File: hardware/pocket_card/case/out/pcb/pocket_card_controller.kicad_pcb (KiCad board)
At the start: 2 copper layers, 80.5 x 37 mm, 19 parts, among them U1 SOIC-28W_7.5x17.9mm_P1.27mm

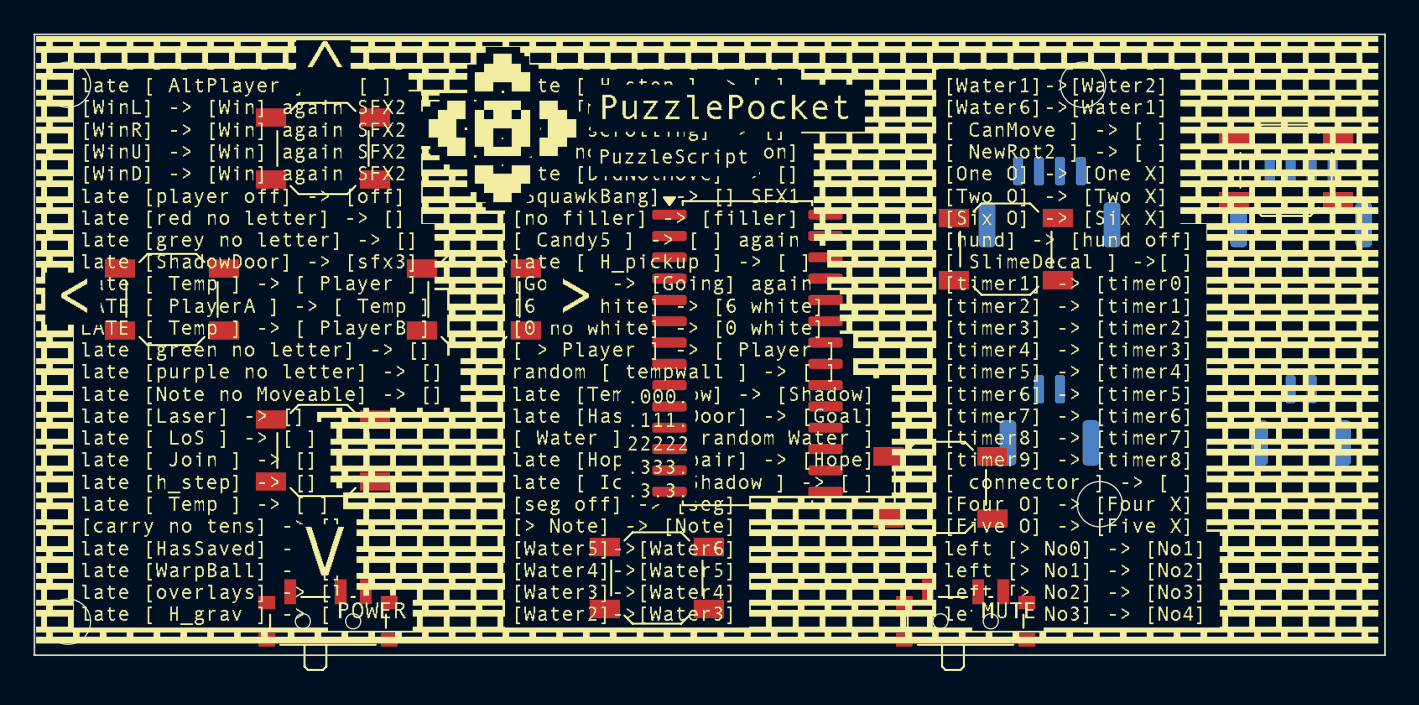
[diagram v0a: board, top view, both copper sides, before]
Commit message: regen pcb
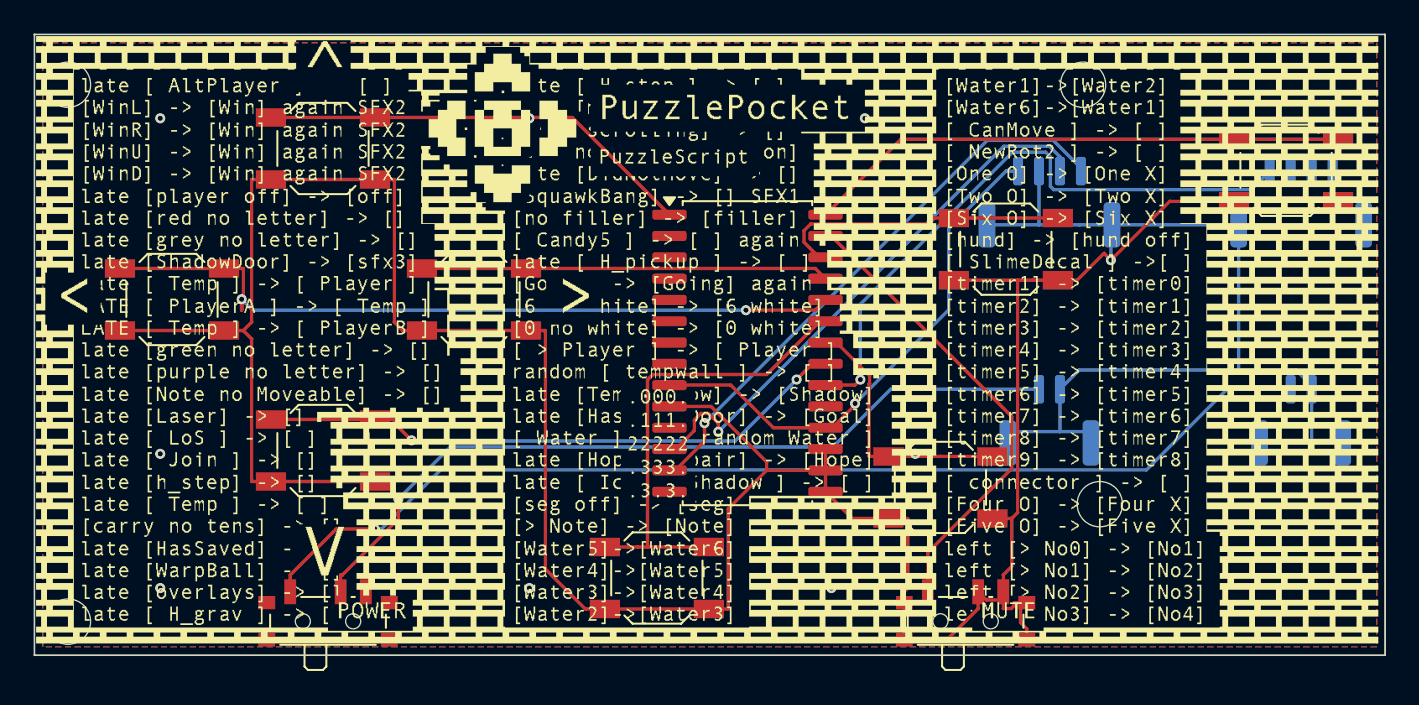
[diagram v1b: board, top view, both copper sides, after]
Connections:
- J_BAT_IN pad 1: (no net) -> BAT_P
- J_BAT_IN pad 2: (no net) -> GND
- J_BAT_IN pad MP: (no net) -> GND
- J_BAT_OUT pad 1: (no net) -> BAT_SW
- J_BAT_OUT pad 2: (no net) -> GND
- J_BAT_OUT pad MP: (no net) -> GND
- J_EXP pad 1: (no net) -> INT
- J_EXP pad MP: (no net) -> GND
- J_I2C pad 1: (no net) -> +3V3
- J_I2C pad 2: (no net) -> GND
- J_I2C pad 3: (no net) -> SCL
- J_I2C pad 4: (no net) -> SDA
- J_I2C pad MP: (no net) -> GND
- SW_ACTION pad 1: (no net) -> SIG_ACTION
- SW_ACTION pad 2: (no net) -> GND
- SW_DOWN pad 1: (no net) -> SIG_DOWN
- SW_DOWN pad 2: (no net) -> GND
- SW_LEFT pad 1: (no net) -> SIG_LEFT
- SW_LEFT pad 2: (no net) -> GND
- SW_MENU pad 1: (no net) -> SIG_MENU
- SW_MENU pad 2: (no net) -> GND
- SW_MUTE pad : (no net) -> GND
- SW_MUTE pad 1: (no net) -> SIG_MUTE
- SW_MUTE pad 2: (no net) -> GND
- SW_MUTE pad 3: (no net) -> GND
- SW_PWR pad 1: (no net) -> BAT_SW
- SW_PWR pad 2: (no net) -> BAT_P
- SW_RESET pad 1: (no net) -> SIG_RESET
- SW_RESET pad 2: (no net) -> GND
- SW_RIGHT pad 1: (no net) -> SIG_RIGHT
- SW_RIGHT pad 2: (no net) -> GND
- SW_UNDO pad 1: (no net) -> SIG_UNDO
- SW_UNDO pad 2: (no net) -> GND
- SW_UP pad 1: (no net) -> SIG_UP
- SW_UP pad 2: (no net) -> GND
- U1 pad 1: (no net) -> SIG_UP
- U1 pad 10: (no net) -> GND
- U1 pad 12: (no net) -> SCL
- U1 pad 13: (no net) -> SDA
- U1 pad 15: (no net) -> GND
- U1 pad 16: (no net) -> GND
- U1 pad 17: (no net) -> GND
- U1 pad 18: (no net) -> +3V3
- U1 pad 20: (no net) -> INT
- U1 pad 21: (no net) -> SIG_DOWN
- U1 pad 22: (no net) -> SIG_RESET
- U1 pad 23: (no net) -> SIG_MENU
- U1 pad 24: (no net) -> SIG_LEFT
- U1 pad 25: (no net) -> SIG_RIGHT
- U1 pad 26: (no net) -> SIG_UNDO
- U1 pad 27: (no net) -> SIG_MUTE
- U1 pad 28: (no net) -> SIG_ACTION
- U1 pad 9: (no net) -> +3V3
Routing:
- net GND: track 0.00 -> 248.4 mm, vias 0 -> 7
- net BAT_SW: track 0.00 -> 65.2 mm, vias 0 -> 1
- net BAT_P: track 0.00 -> 48.0 mm, vias 0 -> 1
- net SIG_LEFT: track 0.00 -> 47.2 mm, vias 0 -> 2
- net INT: track 0.00 -> 37.3 mm, vias 0 -> 1
- net SIG_DOWN: track 0.00 -> 36.3 mm, vias 0 -> 2
- net SCL: track 0.00 -> 34.6 mm, vias 0 -> 1
- net SDA: track 0.00 -> 34.5 mm, vias 0 -> 1
- net SIG_ACTION: track 0.00 -> 32.4 mm
- net +3V3: track 0.00 -> 31.1 mm, vias 0 -> 1
- net SIG_MENU: track 0.00 -> 28.2 mm
- net SIG_MUTE: track 0.00 -> 28.1 mm
- net SIG_UP: track 0.00 -> 26.2 mm, vias 0 -> 1
- net SIG_RIGHT: track 0.00 -> 24.3 mm
- net SIG_UNDO: track 0.00 -> 17.8 mm
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- added copper zone on B.Cu, net GND
- added copper zone on F.Cu, net GND
